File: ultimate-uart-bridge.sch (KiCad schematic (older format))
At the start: 20 parts, among them J101 USB_B_Micro, J102 Conn_01x03, J103 Conn_01x03

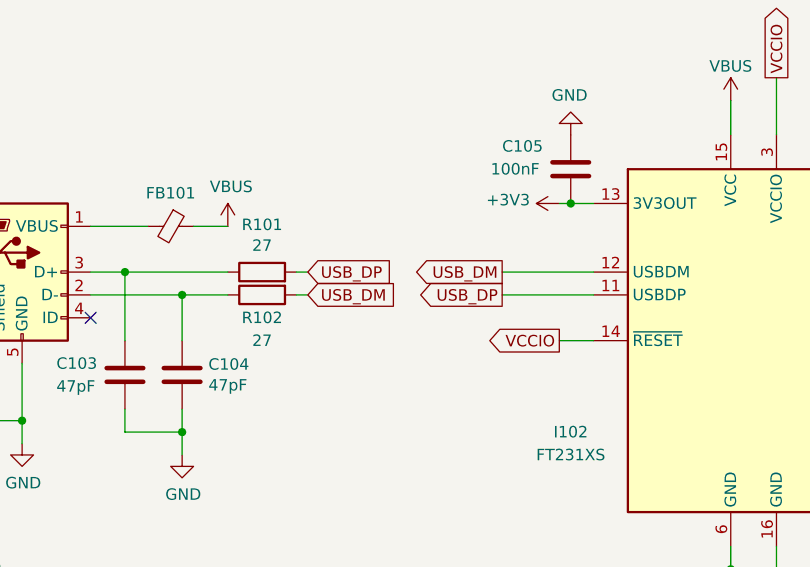
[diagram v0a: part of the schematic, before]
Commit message: First Routing
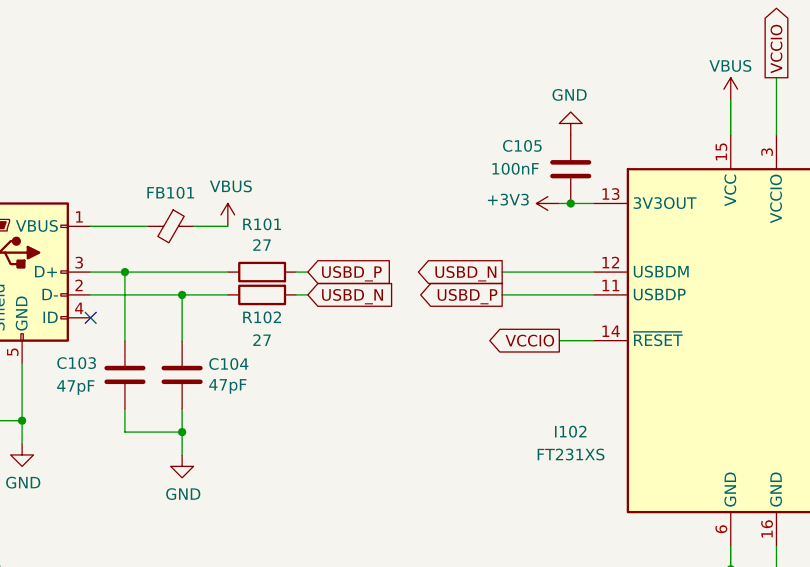
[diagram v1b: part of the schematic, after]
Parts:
- FB101: footprint Filter:Filter_1411-5_1.4x1.1mm -> Ferrite_THT:LairdTech_28C0236-0JW-10
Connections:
- net USB_DM renamed USBD_N
- net USB_DP renamed USBD_P
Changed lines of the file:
@@
 $EndComp
 Text GLabel 3450 3450 2    50   Input ~ 0
-USB_DP
+USBD_P
 Text GLabel 3450 3550 2    50   Input ~ 0
-USB_DM
+USBD_N
 Wire Wire Line
 	2500 3450 2650 3450
 Text GLabel 4300 3550 0    50   Output ~ 0
-USB_DP
+USBD_P
 Text GLabel 4300 3450 0    50   Output ~ 0
-USB_DM
+USBD_N
 Wire Wire Line
 	4300 3450 4700 3450
@@
 F 0 "FB101" V 2705 3250 50  0000 C CNN
 F 1 "Ferrite_Bead_Small" V 2704 3250 50  0001 C CNN
-F 2 "Filter:Filter_1411-5_1.4x1.1mm" V 2780 3250 50  0001 C CNN
+F 2 "Ferrite_THT:LairdTech_28C0236-0JW-10" V 2780 3250 50  0001 C CNN
 F 3 "~" H 2850 3250 50  0001 C CNN
 	1    2850 3250

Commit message: Change Switch Circuit
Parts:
- removed J101: USB_B_Micro, Connector_USB:USB_Micro-B_Molex_47346-0001, symbol Connector:USB_B_Micro
- removed J102: Conn_01x03, Connector_PinHeader_2.54mm:PinHeader_1x03_P2.54mm_Vertical, symbol Connector_Generic:Conn_01x03
- added J101: Conn_02x03_Row_Letter_First, Connector_PinHeader_2.54mm:PinHeader_2x03_P2.54mm_Vertical_SMD, symbol Connector_Generic:Conn_02x03_Row_Letter_First
- added J102: USB_C_Receptacle_USB2.0, Connector_USB:USB_C_Receptacle_GCT_USB4085, symbol Connector:USB_C_Receptacle_USB2.0
- added R105, R106: 5.1k, symbol Device:R_US
- J103: footprint Connector_PinHeader_2.54mm:PinHeader_1x03_P2.54mm_Horizontal -> Connector_PinHeader_2.54mm:PinHeader_1x03_P2.54mm_Vertical_SMD_Pin1Left
- R101, R102, R103, R104: symbol Device:R -> Device:R_US
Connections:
- net +1V8: now also J101.b3 (Pin_b3)
- net +3V3: now also D101.2 (A), D102.2 (A), J101.b2 (Pin_b2)
- net GND: now also J102.A1 (GND), J102.A12 (GND), J102.B1 (GND), J102.B12 (GND), J102.S1 (SHIELD), R105.1, R106.2
- net VBUS: now also J101.b1 (Pin_b1)
- net VCCIO: now also J101.a1 (Pin_a1), J101.a2 (Pin_a2), J101.a3 (Pin_a3); no longer D101.2 (A), D102.2 (A)
- net at FB101.2: now also J102.A4 (VBUS), J102.A9 (VBUS), J102.B4 (VBUS), J102.B9 (VBUS)
- net at R102.1: now also C103.1, J102.A7 (D-), J102.B7 (D-); no longer C104.1
- net at R101.1: now also C104.1, J102.A6 (D+), J102.B6 (D+); no longer C103.1
- new net: J102.A5 (CC1), R105.2
- new net: J102.B5 (CC2), R106.1
- no-connect marks 9 -> 10
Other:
- moved on the sheet: C103, C104, FB101

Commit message: Update Ferrite Bead
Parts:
- FB101: footprint Ferrite_THT:LairdTech_28C0236-0JW-10 -> Inductor_SMD:L_0805_2012Metric_Pad1.15x1.40mm_HandSolder; PartNo (none) -> MI0805K400R-10
- R105, R106: footprint (none) -> Resistor_SMD:R_0805_2012Metric_Pad1.20x1.40mm_HandSolder
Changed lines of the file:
@@
 F 0 "FB101" V 2205 2700 50  0000 C CNN
 F 1 "Ferrite_Bead_Small" V 2204 2700 50  0001 C CNN
-F 2 "Ferrite_THT:LairdTech_28C0236-0JW-10" V 2280 2700 50  0001 C CNN
+F 2 "Inductor_SMD:L_0805_2012Metric_Pad1.15x1.40mm_HandSolder" V 2280 2700 50  0001 C CNN
 F 3 "~" H 2350 2700 50  0001 C CNN
+F 4 "MI0805K400R-10" V 2350 2700 50  0001 C CNN "PartNo"
 	1    2350 2700
 	0    1    1    0
@@
 F 0 "R105" V 2100 2800 50  0000 C CNN
 F 1 "5.1k" V 2100 3000 50  0000 C CNN
-F 2 "" V 2240 2890 50  0001 C CNN
+F 2 "Resistor_SMD:R_0805_2012Metric_Pad1.20x1.40mm_HandSolder" V 2240 2890 50  0001 C CNN
 F 3 "~" H 2200 2900 50  0001 C CNN
 	1    2200 2900
@@
 F 0 "R106" V 2100 3100 50  0000 C CNN
 F 1 "5.1k" V 2100 2900 50  0000 C CNN
-F 2 "" V 2240 2990 50  0001 C CNN
+F 2 "Resistor_SMD:R_0805_2012Metric_Pad1.20x1.40mm_HandSolder" V 2240 2990 50  0001 C CNN
 F 3 "~" H 2200 3000 50  0001 C CNN
 	1    2200 3000
